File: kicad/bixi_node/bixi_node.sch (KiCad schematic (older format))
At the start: 6 parts, among them J1 RJ45, P1 CONN_01X03, U1 SP3485CN

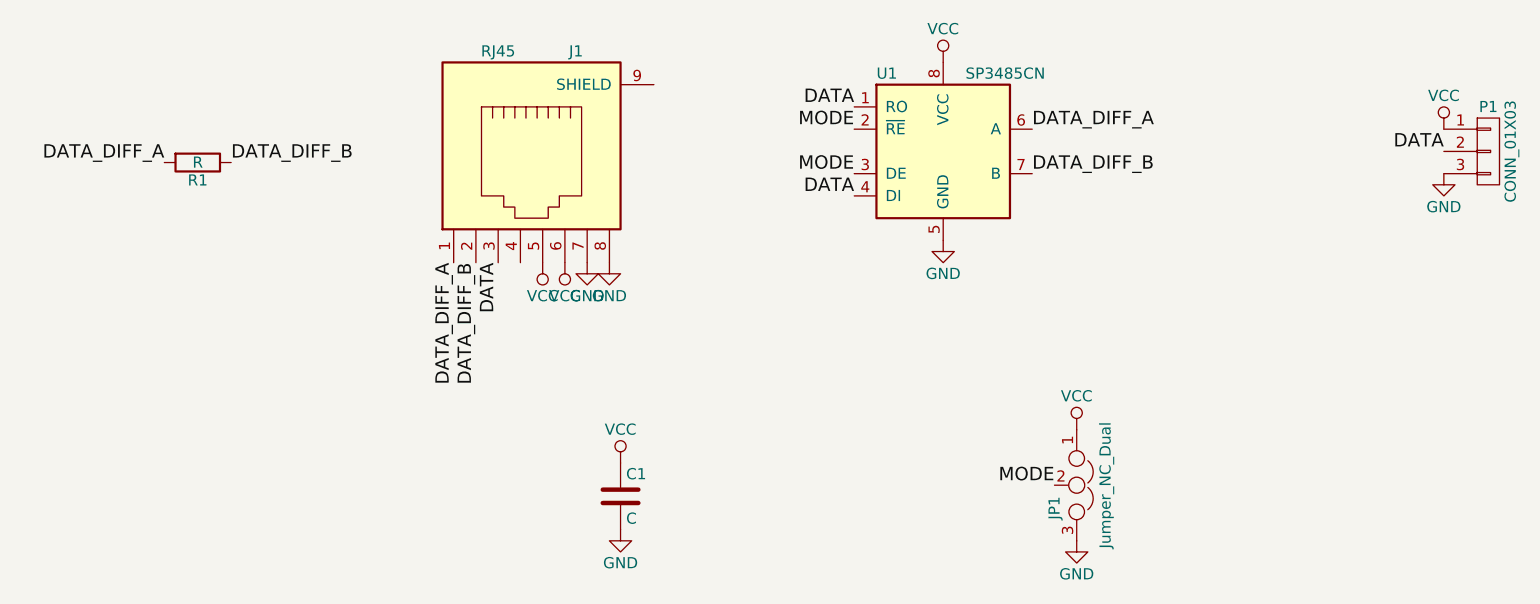
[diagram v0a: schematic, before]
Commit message: v3 pcb's plotted, ready for fab
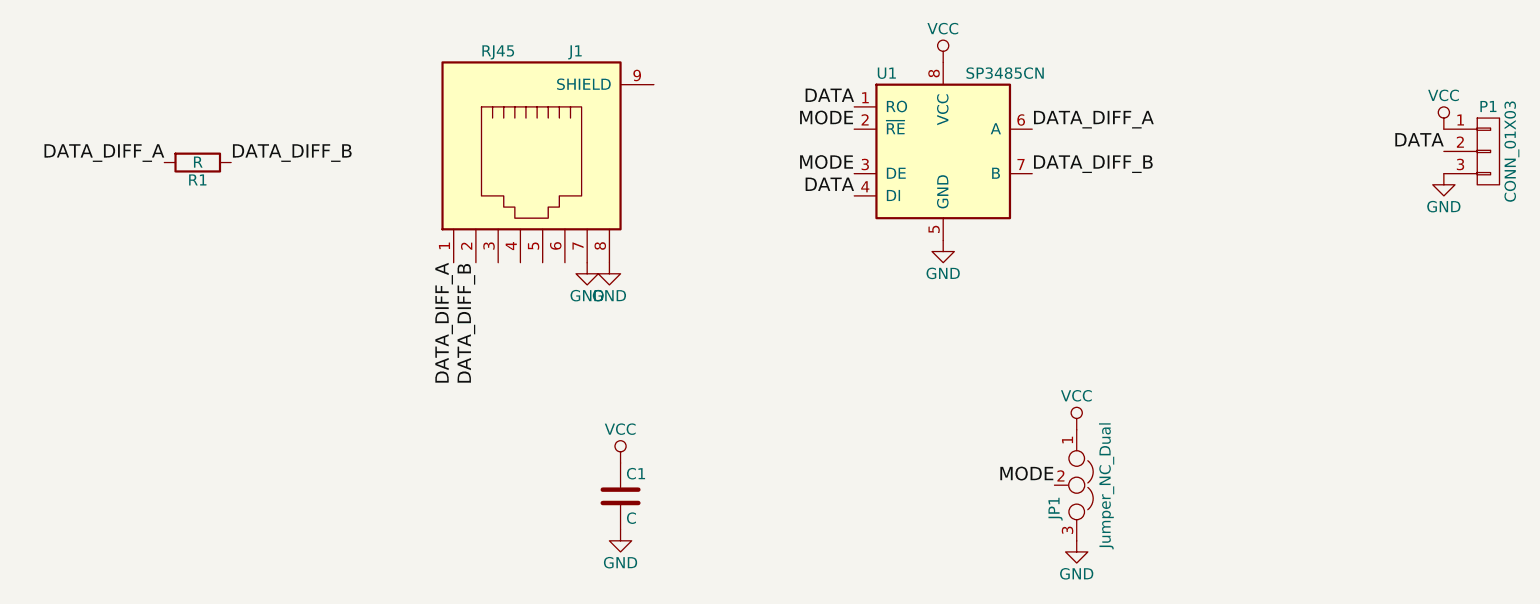
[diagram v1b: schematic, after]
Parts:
- P1: footprint Connectors_JST:JST_EH_S03B-EH_03x2.50mm_Angled -> custom:PAD_3X_OVAL_WS2812B
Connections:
- net DATA: no longer J1.3
- net VCC: no longer J1.5, J1.6
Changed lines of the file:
@@
 F 0 "P1" H 8250 3500 50  0000 C CNN
 F 1 "CONN_01X03" V 8350 3300 50  0000 C CNN
-F 2 "Connectors_JST:JST_EH_S03B-EH_03x2.50mm_Angled" H 8250 3300 50  0001 C CNN
+F 2 "custom:PAD_3X_OVAL_WS2812B" H 8250 3300 50  0001 C CNN
 F 3 "" H 8250 3300 50  0000 C CNN
 	1    8250 3300
@@
 $EndComp
 $Comp
-L VCC #PWR011
+L VCC #PWR09
 U 1 1 58EA51F3
 P 6400 4550
-F 0 "#PWR011" H 6400 4400 50  0001 C CNN
+F 0 "#PWR09" H 6400 4400 50  0001 C CNN
 F 1 "VCC" H 6400 4700 50  0000 C CNN
 F 2 "" H 6400 4550 50  0000 C CNN
@@
 $EndComp
 $Comp
-L GND #PWR012
+L GND #PWR010
 U 1 1 58EA5217
 P 6400 5050
-F 0 "#PWR012" H 6400 4800 50  0001 C CNN
+F 0 "#PWR010" H 6400 4800 50  0001 C CNN
 F 1 "GND" H 6400 4900 50  0000 C CNN
 F 2 "" H 6400 5050 50  0000 C CNN
@@
 Text Label 3700 3800 3    60   ~ 0
 DATA_DIFF_B
-Text Label 3800 3800 3    60   ~ 0
-DATA
 Text Label 2300 3350 2    60   ~ 0
 DATA_DIFF_A
@@
 Text Label 6300 4800 2    60   ~ 0
 MODE
-$Comp
-L VCC #PWR013
-U 1 1 5902A84B
-P 4100 3800
-F 0 "#PWR013" H 4100 3650 50  0001 C CNN
-F 1 "VCC" H 4100 3950 50  0000 C CNN
-F 2 "" H 4100 3800 50  0000 C CNN
-F 3 "" H 4100 3800 50  0000 C CNN
-	1    4100 3800
-	-1   0    0    1
-$EndComp
-$Comp
-L VCC #PWR014
-U 1 1 5902A94D
-P 4000 3800
-F 0 "#PWR014" H 4000 3650 50  0001 C CNN
-F 1 "VCC" H 4000 3950 50  0000 C CNN
-F 2 "" H 4000 3800 50  0000 C CNN
-F 3 "" H 4000 3800 50  0000 C CNN
-	1    4000 3800
-	-1   0    0    1
-$EndComp
 $EndSCHEMATC
